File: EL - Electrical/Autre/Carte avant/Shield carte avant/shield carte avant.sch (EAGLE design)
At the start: 14 parts, among them J5 22-05-7028-02

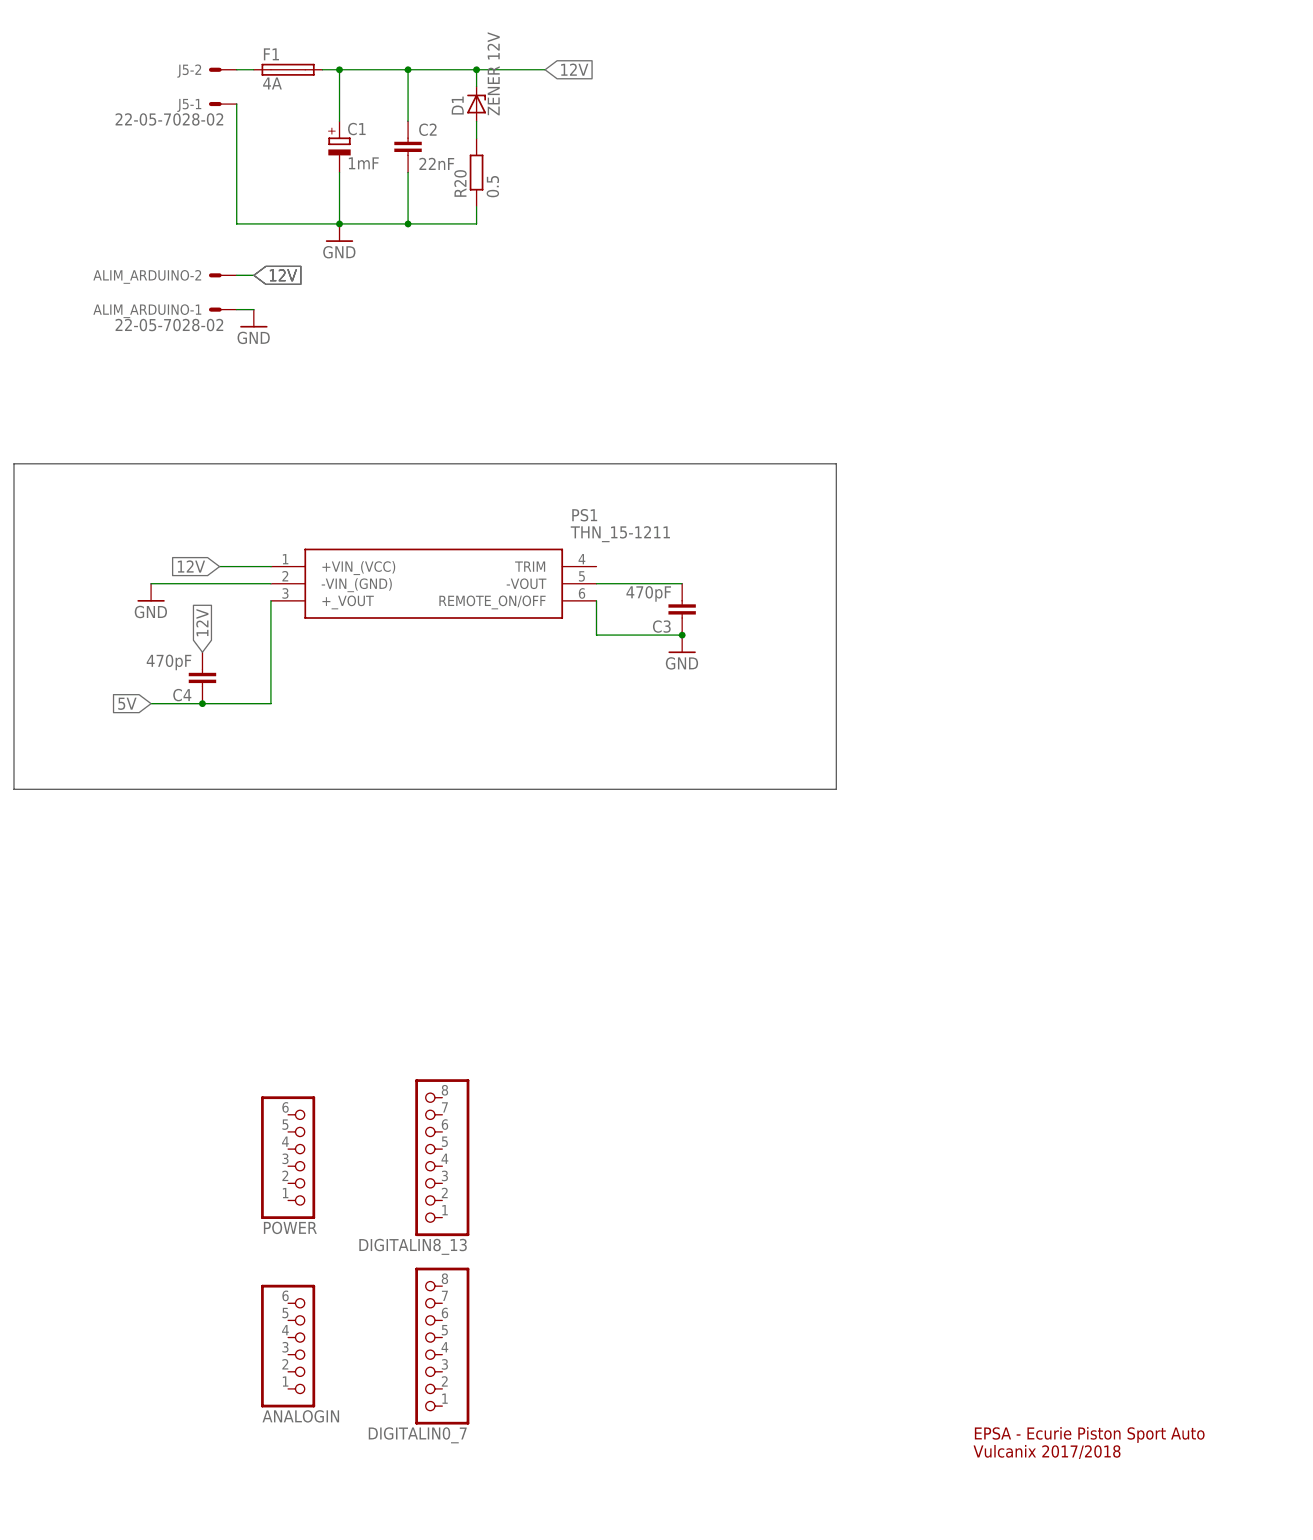
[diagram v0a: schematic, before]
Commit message: shield carte avant
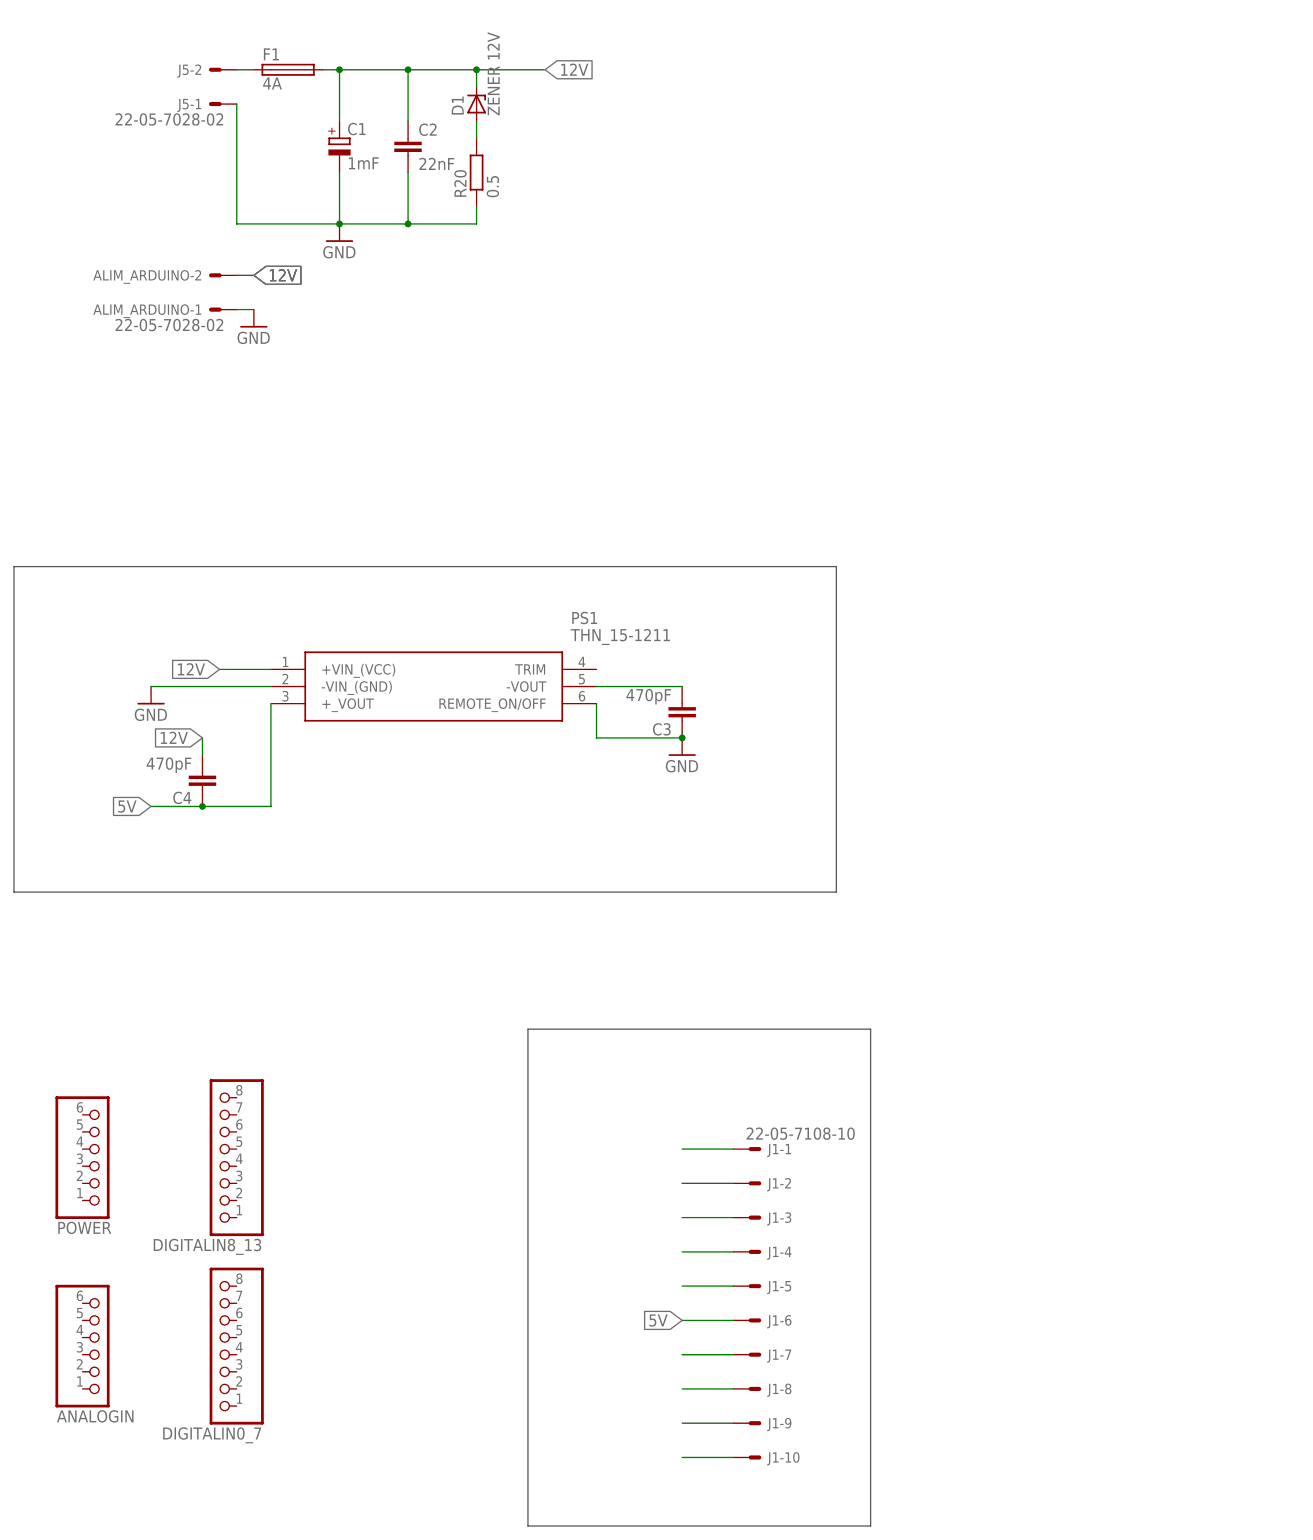
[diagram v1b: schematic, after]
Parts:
- added J1: 22-05-7108-10, con-molex:22-05-7108-10
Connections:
- new net N$11: J1-7.S
- new net N$12: J1-8.S
- new net N$13: J1-9.S
- new net N$14: J1-10.S
- new net N$6: J1-2.S
- new net N$7: J1-3.S
- new net N$8: J1-4.S
- new net N$9: J1-5.S
- net 12V: now also C4.2
- net 5V: now also J1-1.S, J1-6.S
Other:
- note removed: "EPSA - Ecurie Piston Sport Auto Vulcanix 2017/2018"
- moved on the sheet: ANALOGIN, C3, C4, DIGITALIN0_7, DIGITALIN8_13, POWER, PS1
